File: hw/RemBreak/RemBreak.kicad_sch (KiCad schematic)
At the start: 5 parts, among them J2 Conn_02x06_Odd_Even, J3 Screw_Terminal_01x04, J5 Screw_Terminal_01x04

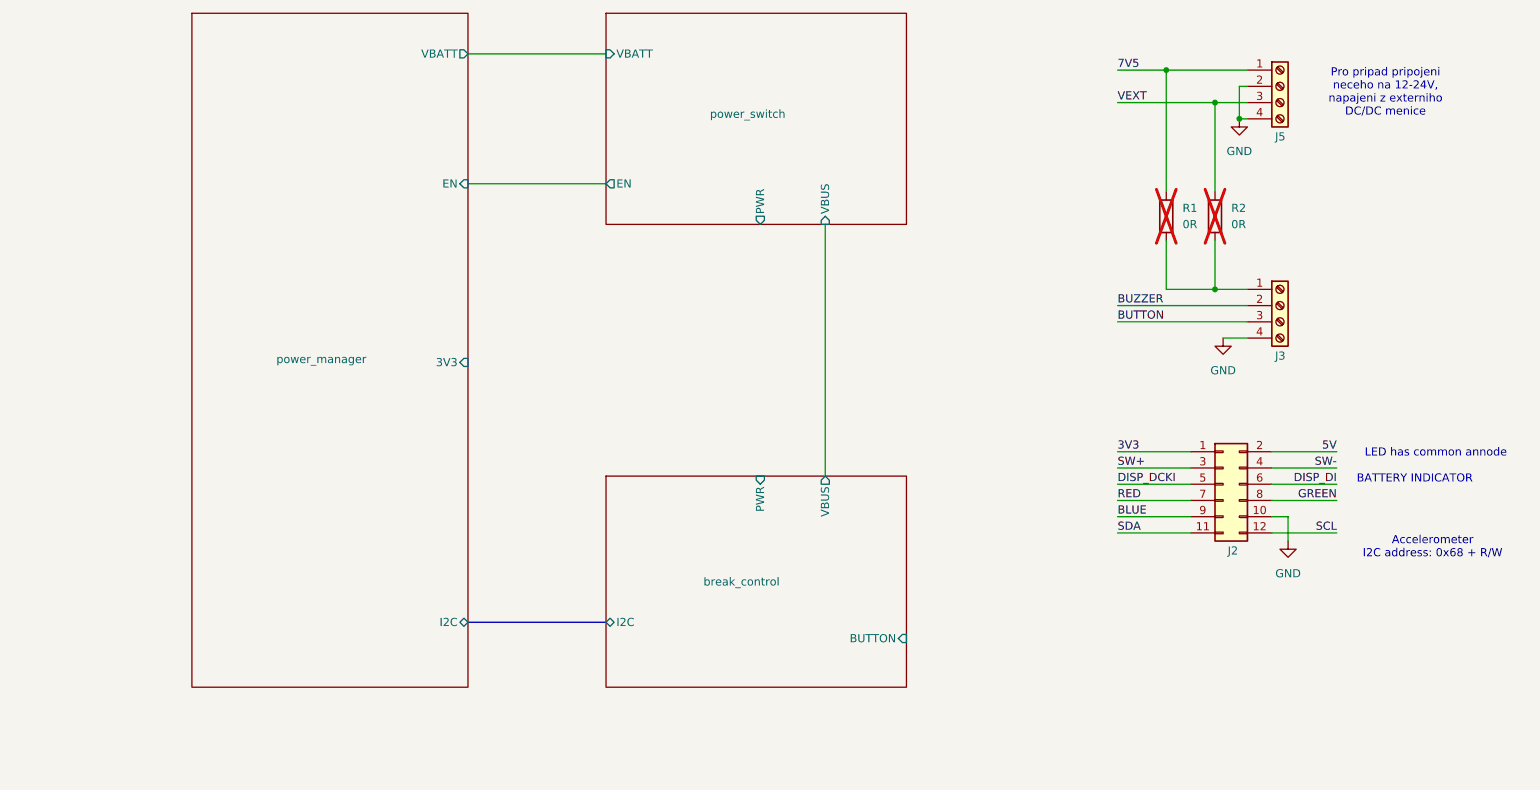
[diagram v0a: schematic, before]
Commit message: finished schematics routing and erc passed
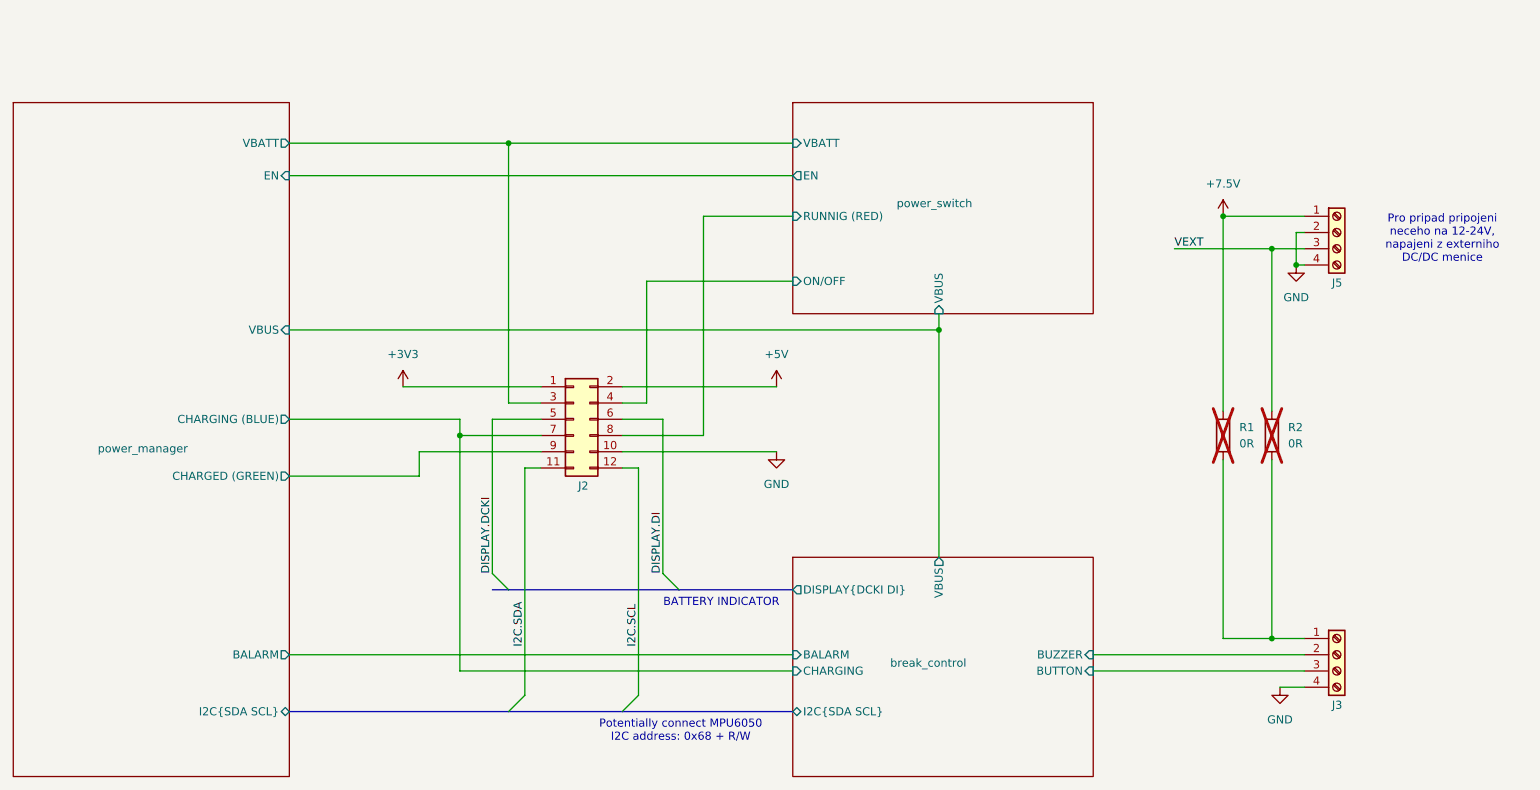
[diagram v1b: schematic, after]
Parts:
- J2: footprint dodo_conn:SAMTEC_TSM-106-01-L-DH-P-TR -> chinese_modules:SAMTEC_TSM-106-01-L-DH-P-TR
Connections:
- net BUTTON is gone; now on net break_control/BUTTON: J3.3 (Pin_3)
- net SW+ is gone; now on net power_manager/VBATT: J2.3 (Pin_3)
- net 3V3 renamed +3V3
- net 5V renamed +5V
- net 7V5 renamed +7.5V
- net BLUE renamed power_manager/CHARGED (GREEN)
- net BUZZER renamed break_control/BUZZER
- net DISP_DCKI renamed DISPLAY.DCKI
- net DISP_DI renamed DISPLAY.DI
- net GREEN renamed power_switch/RUNNIG (RED)
- net RED renamed break_control/CHARGING
- net SCL renamed I2C.SCL
- net SDA renamed I2C.SDA
- net SW- renamed power_switch/ON/OFF
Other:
- sheet break_control ports: added BALARM, BUZZER, CHARGING, DISPLAY{DCKI DI}, I2C{SDA SCL}; removed I2C, PWR
- sheet power_manager ports: added BALARM, CHARGED (GREEN), CHARGING (BLUE), I2C{SDA SCL}, VBUS; removed 3V3, I2C
- sheet power_switch ports: added ON/OFF, RUNNIG (RED); removed PWR
- note added: "Potentially connect MPU6050 I2C address: 0x68 + R/W"
- note removed: "Accelerometer I2C address: 0x68 + R/W"
- note removed: "LED has common annode"
- moved on the sheet: J2, J3, J5, R1, R2
